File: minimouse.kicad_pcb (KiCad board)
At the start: 2 copper layers, 90 x 85 mm, 50 parts, among them J1 Conn_ARM_JTAG_SWD_10, J4 Conn_01x04_Pin, J5 Conn_01x02, J6 Conn_01x06, J7 Conn_01x06, M1 N20_encoder, M2 N20_encoder, U1 STM32F030C8Tx, U3 LP5907MFX-1.2, U4 HC-SR04, U5 STSPIN240

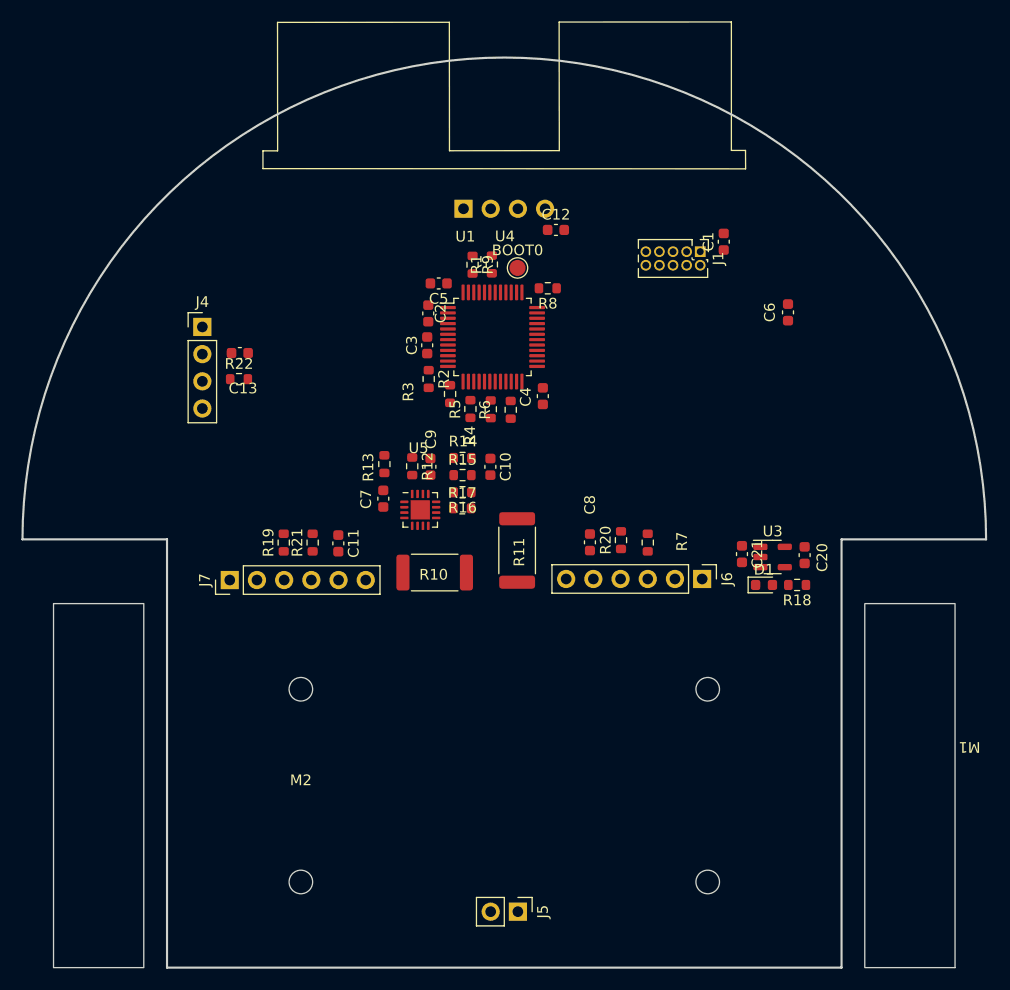
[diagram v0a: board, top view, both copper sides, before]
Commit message: version6
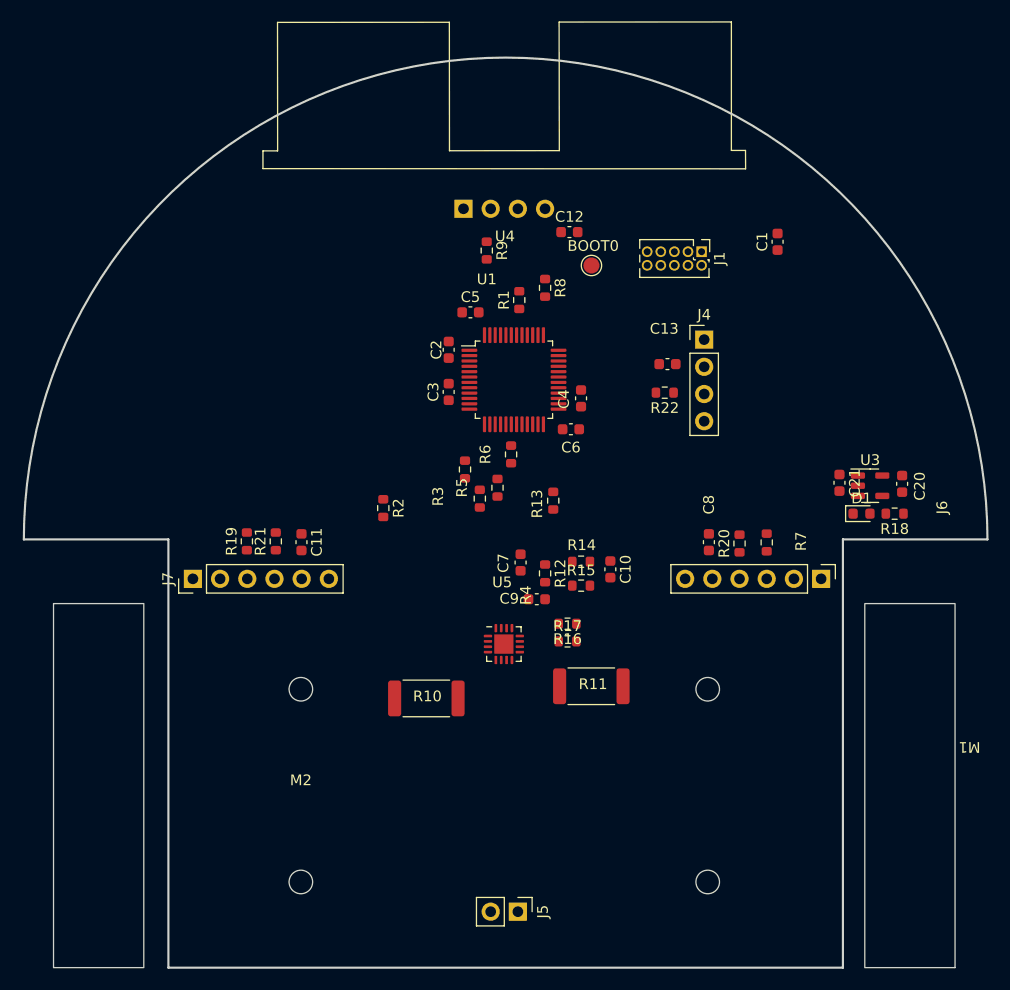
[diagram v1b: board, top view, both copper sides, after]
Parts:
- moved J4 46.9 mm to (168.7, 81.3)
- moved C13 40.0 mm to (165.2, 83.6), turned to 0 degrees
- moved R22 39.8 mm to (165.0, 86.3), turned to 180 degrees
- moved C6 23.0 mm to (156.2, 89.7), turned to 0 degrees
- moved R13 16.1 mm to (154.6, 96.4)
- moved R12 15.9 mm to (153.8, 103.2)
- moved C9 15.9 mm to (153.0, 105.6), turned to 180 degrees
- moved R17 15.8 mm to (155.9, 109.5)
- moved R16 15.7 mm to (155.9, 107.9)
- moved R15 15.1 mm to (157.2, 104.3)
- moved U5 14.8 mm to (150.0, 109.8)
- moved C10 14.7 mm to (159.9, 102.8)
- moved R14 14.7 mm to (157.2, 102.1)
- moved R11 14.5 mm to (158.1, 113.7), turned to 0 degrees
- moved C7 14.1 mm to (151.5, 102.2)
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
